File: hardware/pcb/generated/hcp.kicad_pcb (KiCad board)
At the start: 2 copper layers, 65 x 44.5 mm, 9 parts, among them J1 HCP2 6P6C, U1 ESP32-C3 Super Mini, U2 Isolated RS485

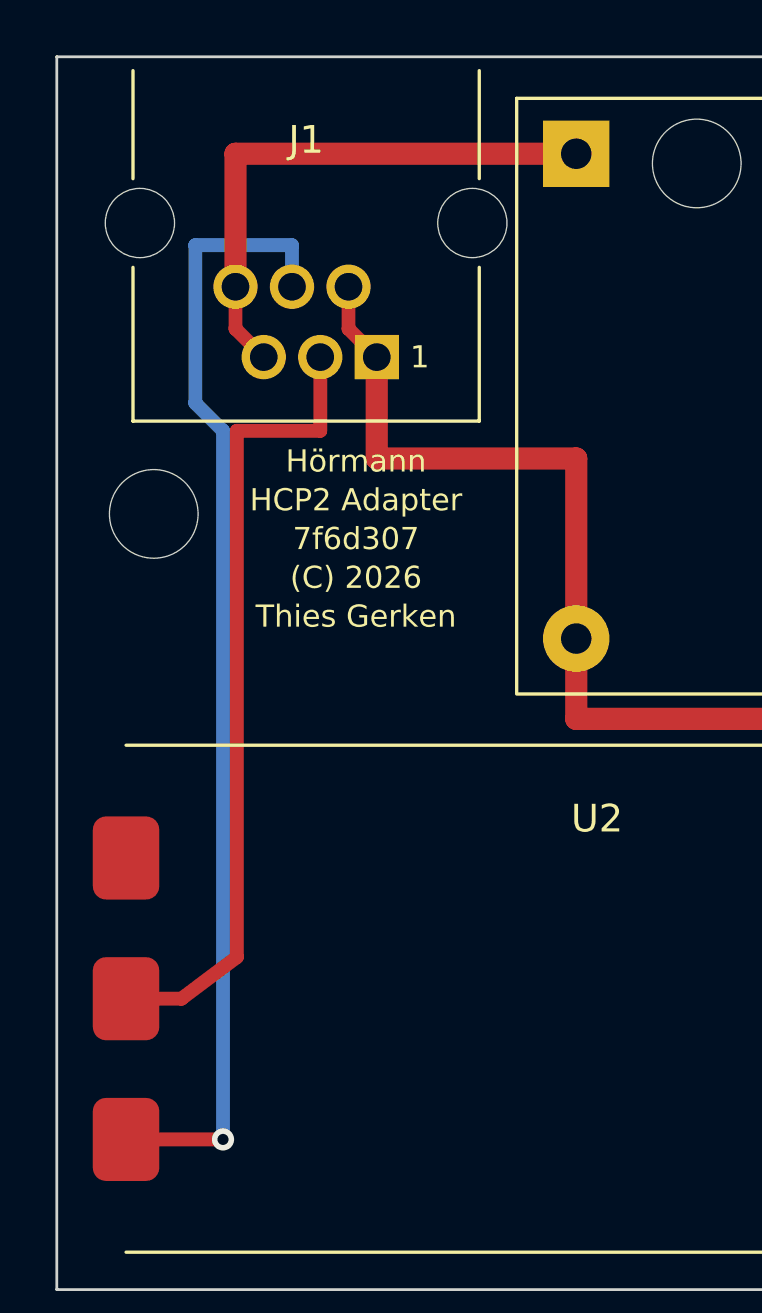
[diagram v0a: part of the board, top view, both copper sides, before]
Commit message: Regenerate outputs
Co-Authored-By: Claude Fable 5.1 <noreply@anthropic.com>
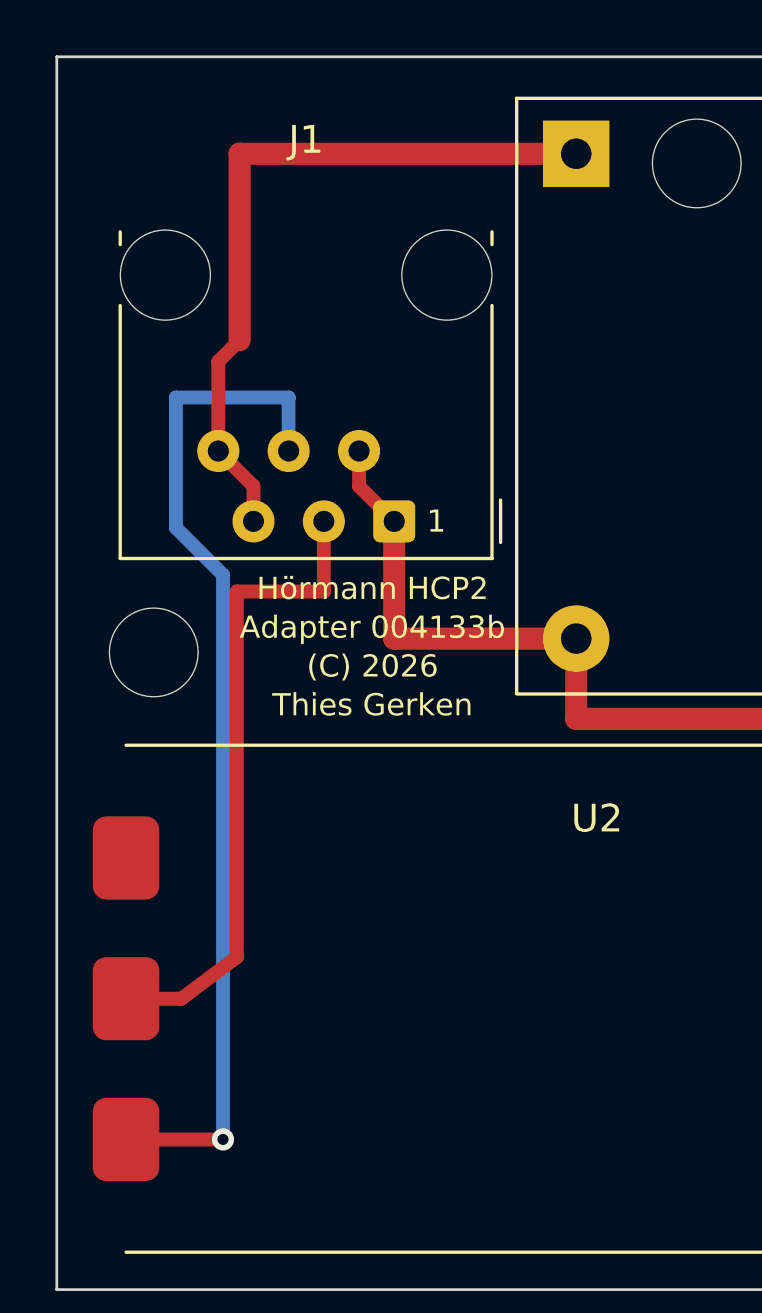
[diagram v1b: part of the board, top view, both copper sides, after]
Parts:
- J1: footprint HCP:RJ12_95001_6P6C -> HCP:RJ12_Amphenol_54601-x06_Horizontal
- moved J1 17.1 mm to (128.2, 84.8), turned to 180 degrees
- moved H1 5.00 mm to (119.5, 89.5)
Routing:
- net HCP_GND: track 105.4 -> 98.9 mm
- net HCP_25V: track 20.1 -> 26.3 mm
- net HCP_B_MINUS: track 29.2 -> 23.4 mm
- net HCP_A_PLUS: track 41.2 -> 37.0 mm
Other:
- board text added: "Adapter 004133b"
- board text added: "Hörmann HCP2"
- board text removed: "7f6d307"
- board text removed: "HCP2 Adapter"
- board text removed: "Hörmann"
